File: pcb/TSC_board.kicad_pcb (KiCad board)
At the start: 4 copper layers, 100 x 100 mm, 427 parts, among them IC1 TS3021ILT, IC10 TS3021ILT, IC11 TS3021ILT, IC12 TS3021ILT, IC13 TS3021ILT, IC14 TS3021ILT, IC15 NCP51460SN33T1G, IC16 NCP51460SN33T1G, IC17 NCP51460SN33T1G, IC18 NCP51460SN33T1G, IC2 TS3021ILT, IC3 TS3021ILT, IC4 TS3021ILT, IC5 TS3021ILT, IC6 TS3021ILT, IC7 TS3021ILT, IC8 TS3021ILT, IC9 TS3021ILT, J1 Conn_01x05_Socket, J2 Conn_01x05_Socket, J3 Conn_01x04_Socket, J4 Conn_01x04_Socket, U1 TEA1-0505, U10 ADuM1400xRW, U11 GAQY212GS, U12 GAQY212GS, U13 GAQY212GS, U14 GAQY212GS, U15 LM4040DBZ-5, U16 DAC7311xDCK, U17 ADuM1300xRW, U18 TEA1-0505, U19 GAQY212GS, U2 GAQY212GS, U20 GAQY212GS, U21 GAQY212GS, U22 GAQY212GS, U23 GAQY212GS, U24 GAQY212GS, U25 GAQY212GS, U26 GAQY212GS, U27 ADuM1400xRW, U28 GAQY212GS, U29 GAQY212GS, U3 GAQY212GS, U30 GAQY212GS, U31 GAQY212GS, U32 LM4040DBZ-5, U33 DAC7311xDCK, U34 ADuM1300xRW, U35 TEA1-0505, U36 GAQY212GS, U37 GAQY212GS, U38 GAQY212GS, U39 GAQY212GS, U4 GAQY212GS, U40 GAQY212GS, U41 GAQY212GS, U42 ADuM1300xRW, U43 GAQY212GS, U44 GAQY212GS, U45 GAQY212GS, U46 LM4040DBZ-5, U47 DAC7311xDCK, U48 ADuM1300xRW, U49 TEA1-0505, U5 GAQY212GS, U50 GAQY212GS, U51 GAQY212GS, U52 GAQY212GS, U53 GAQY212GS, U54 GAQY212GS, U55 GAQY212GS, U56 ADuM1300xRW, U57 GAQY212GS, U58 GAQY212GS, U59 GAQY212GS, U6 GAQY212GS, U60 LM4040DBZ-5, U61 DAC7311xDCK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

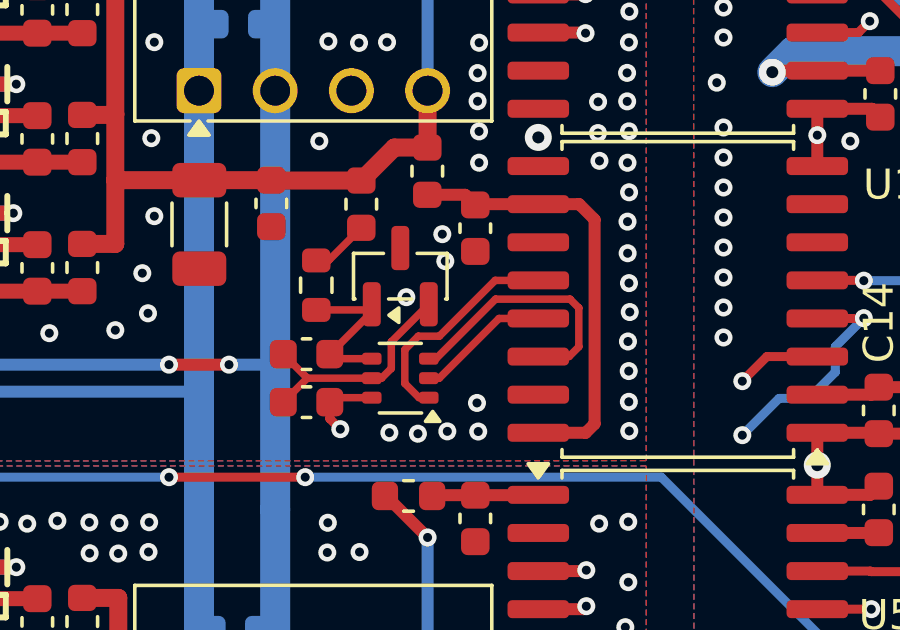
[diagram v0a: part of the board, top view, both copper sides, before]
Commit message: Update dac pwr
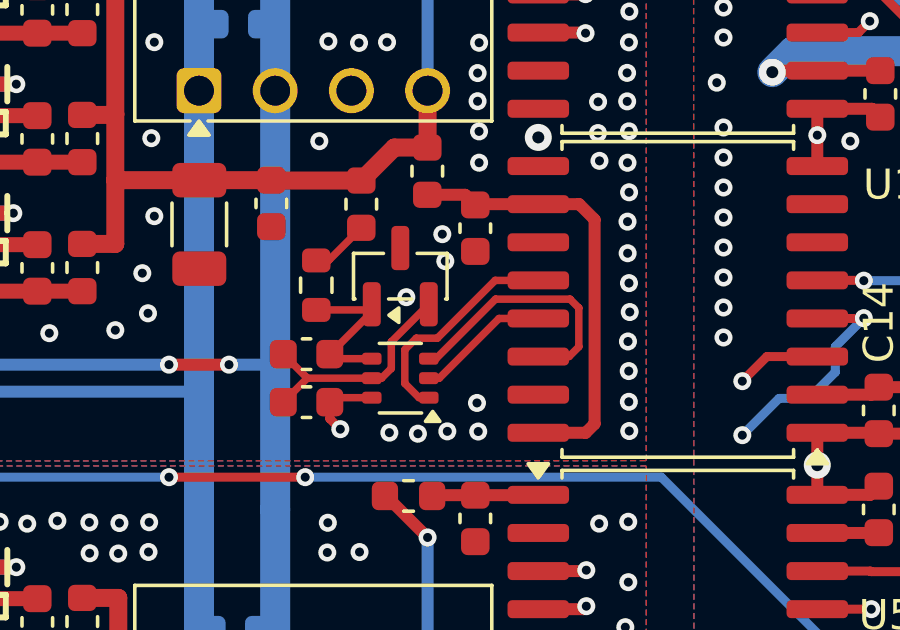
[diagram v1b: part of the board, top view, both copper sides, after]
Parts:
- U32, U46, U60: value LM4040DBZ-5 -> LM4040D33FTA
